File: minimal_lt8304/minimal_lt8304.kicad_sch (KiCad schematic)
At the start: 39 parts, among them J1 FW-02-03-G-D-085-155, J2 FW-02-03-G-D-085-155, J3 FW-02-03-G-D-085-155, J4 FW-02-03-G-D-085-155, T1 750315836, U1 LT8304IS8E-PBF

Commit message: Switch to KiCad 9
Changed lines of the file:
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@@
 (kicad_sch
-	(version 20231120)
+	(version 20250114)
 	(generator "eeschema")
-	(generator_version "8.0")
+	(generator_version "9.0")
 	(paper "A3")
 	(junction
@@
 		)
 	)
+	(embedded_fonts no)
 )

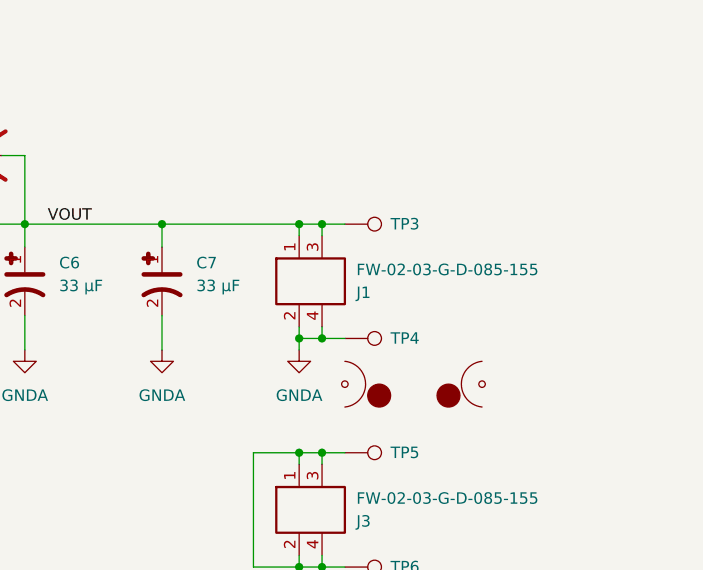
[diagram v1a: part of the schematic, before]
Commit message: Small project update
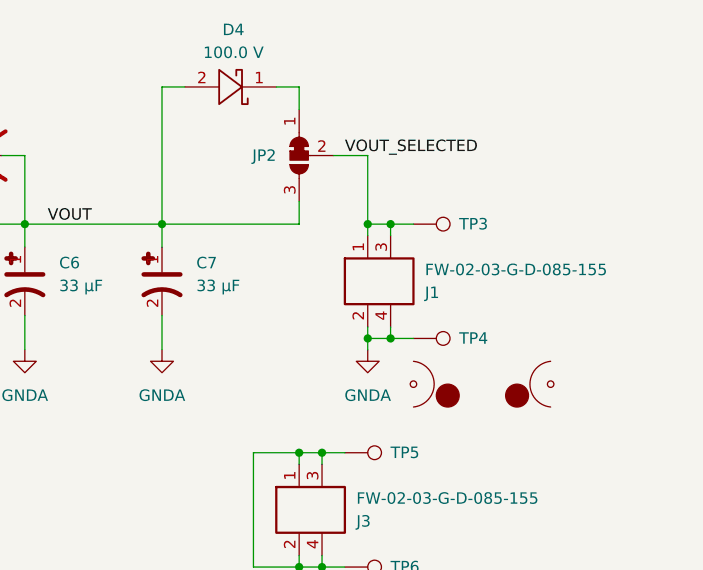
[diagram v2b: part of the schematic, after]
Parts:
- added D4: 100.0 V, diode_footprints:SOD123W, symbol UNITED_DIODES_DATA_BASE:D_PMEG10020AELR
- added JP2: SolderJumper_3_Open, solder_jumper_footprints:SolderJumper-3_P1.3mm_Bridged_1_2_RoundedPad1.0x1.5mm_NumberLabels, symbol UNITED_SOLDER_JUMPERS:SolderJumper_3_Bridged_1_2
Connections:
- net VOUT: now also D4.2, JP2.3 (B); no longer J1.1, J1.3, TP3.1
- new net: D4.1, JP2.1 (A)
- new net VOUT_SELECTED: J1.1, J1.3, JP2.2 (C), TP3.1
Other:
- moved on the sheet: J1, TP3, TP4

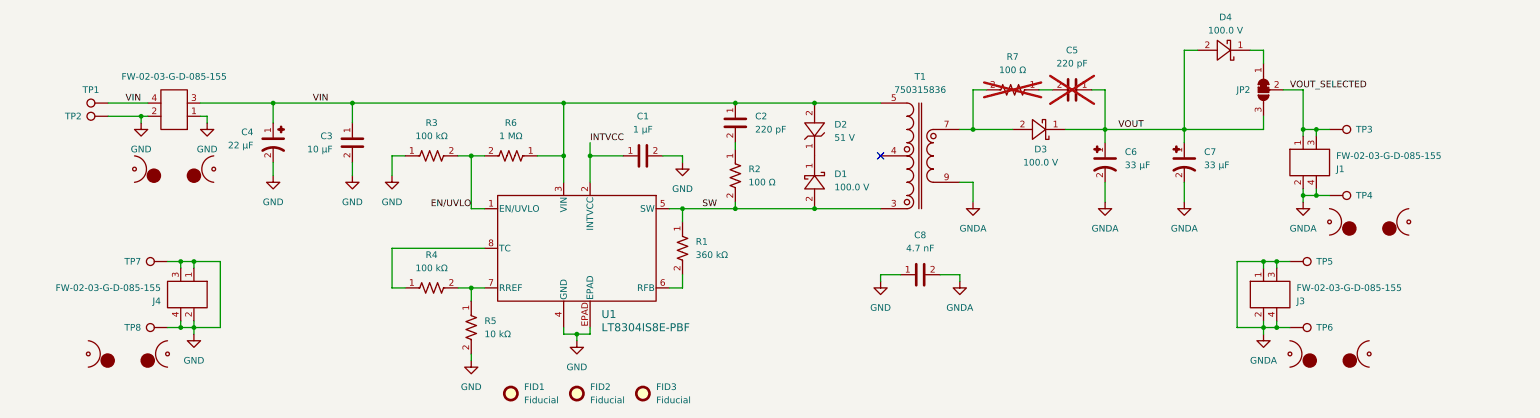
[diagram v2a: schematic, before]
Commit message: update project
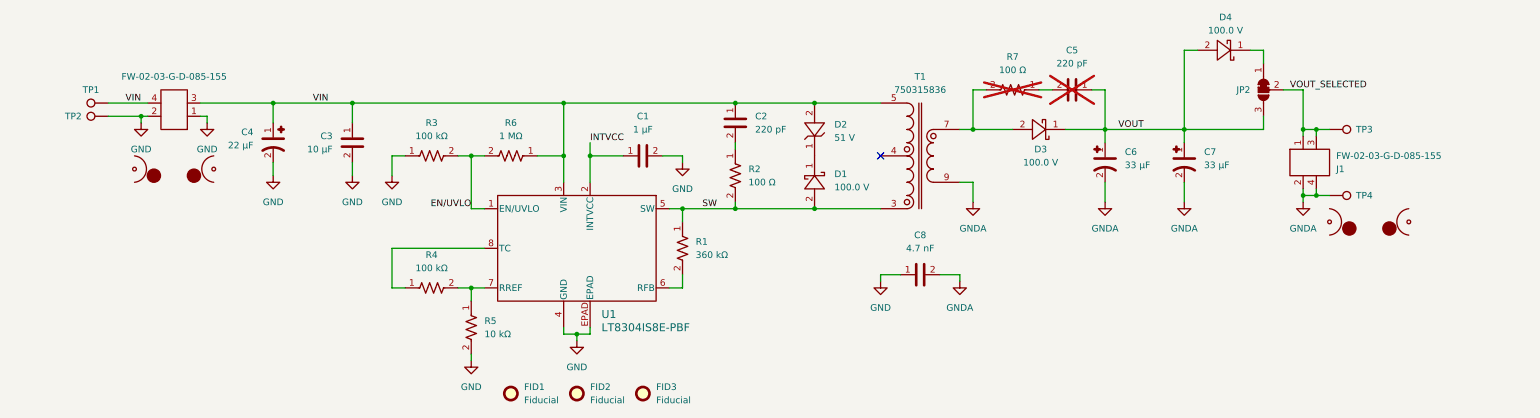
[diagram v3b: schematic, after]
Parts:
- removed J3, J4: FW-02-03-G-D-085-155, connector_footprints:FW-02-03-G-D-085-155, symbol UNITED_CONNECTORS_DATA_BASE:J_FW-02-03-G-D-085-155
- removed MB3, MB4: mouse-bite-midle-50mil-200mil, mouse_bite_footprints:mouse-bite-midle-50mil-200mil, symbol UNITED_MOUSE_BITES_DATA_BASE:mouse-bite-midle-50mil-200mil
- removed TP5, TP6, TP7, TP8: TestPoint, test_point_footprints:TestPoint_THTPad_Castelated, symbol UNITED_TEST_POINTS:TestPoint_Castelated

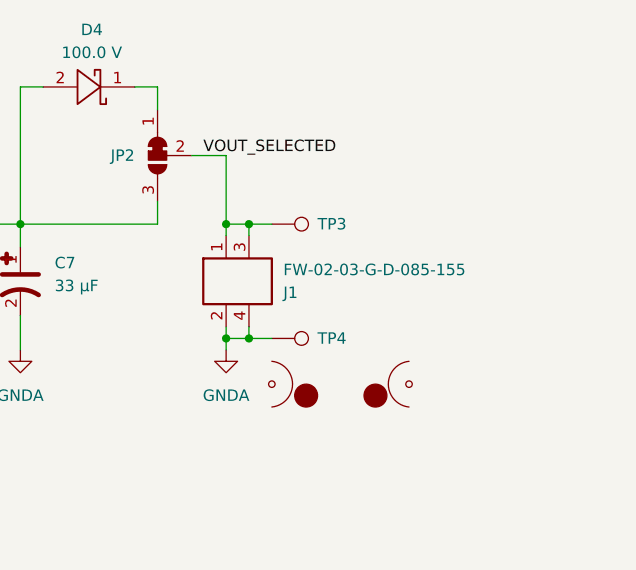
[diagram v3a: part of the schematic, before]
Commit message: development backup
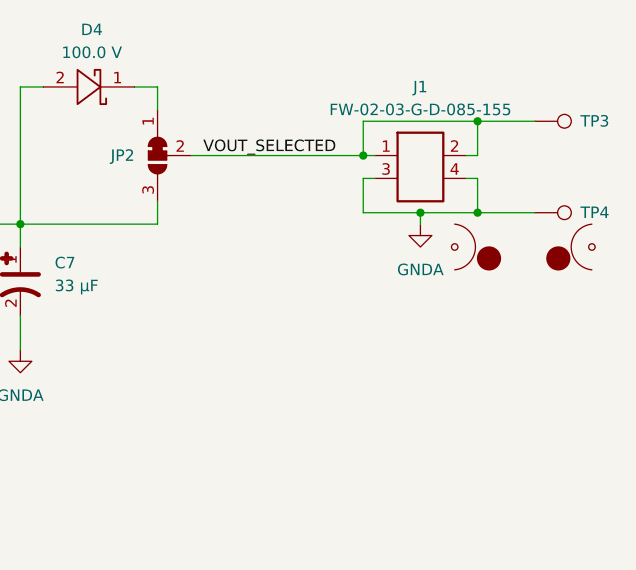
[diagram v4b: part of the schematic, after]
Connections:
- net GNDA: now also J1.3; no longer J1.2
- net VOUT_SELECTED: now also J1.2; no longer J1.3
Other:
- moved on the sheet: J1, TP3, TP4
